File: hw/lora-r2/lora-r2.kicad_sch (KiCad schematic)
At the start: 5 parts, among them J3 Conn_02x12_Odd_Even

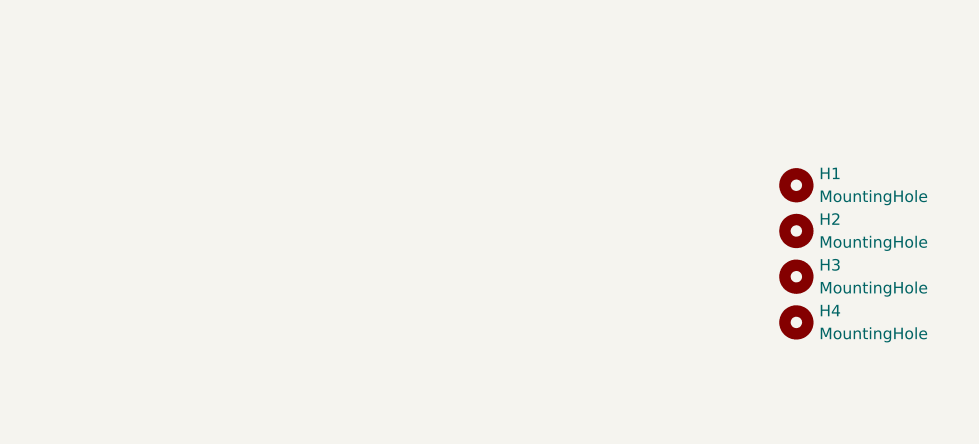
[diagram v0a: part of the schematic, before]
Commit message: Generated first Gerbers
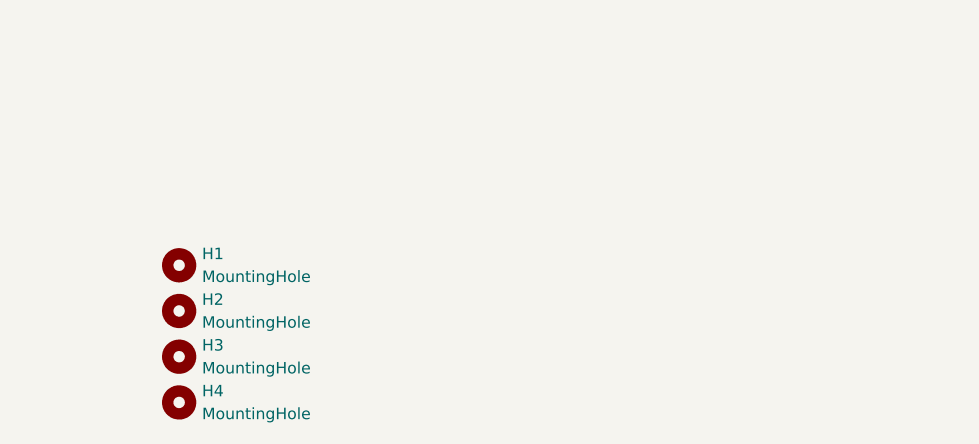
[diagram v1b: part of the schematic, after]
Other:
- company: (none) -> Bruce MacKinnon
- title: (none) -> KC1FSZ LoRa Controller Board
- moved on the sheet: H1, H2, H3, H4
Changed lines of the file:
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@@
 	(generator "eeschema")
 	(generator_version "9.0")
-	(paper "A4")
+	(paper "USLetter")
+	(title_block
+		(title "KC1FSZ LoRa Controller Board")
+		(date "2025-05-08")
+		(rev "1")
+		(company "Bruce MacKinnon")
+		(comment 1 "Copyright (C) 2025, Bruce MacKinnon")
+		(comment 2 "NOT FOR COMMERCIAL USE")
+	)
 	(junction
 		(at 107.95 102.87)
@@
 	(symbol
 		(lib_id "Mechanical:MountingHole")
-		(at 261.62 105.41 0)
+		(at 193.04 114.3 0)
 		(unit 1)
 		(exclude_from_sim yes)
@@
 		(fields_autoplaced yes)
 		(property "Reference" "H4"
-			(at 264.16 104.1399 0)
+			(at 195.58 113.0299 0)
 			(effects
 				(font
@@
 		)
 		(property "Value" "MountingHole"
-			(at 264.16 106.6799 0)
+			(at 195.58 115.5699 0)
 			(effects
 				(font
@@
 		)
 		(property "Footprint" "MountingHole:MountingHole_3.5mm"
-			(at 261.62 105.41 0)
+			(at 193.04 114.3 0)
 			(effects
 				(font
@@
 		)
 		(property "Datasheet" "~"
-			(at 261.62 105.41 0)
+			(at 193.04 114.3 0)
 			(effects
 				(font
@@
 		)
 		(property "Description" "Mounting Hole without connection"
-			(at 261.62 105.41 0)
+			(at 193.04 114.3 0)
 			(effects
 				(font
@@
 	(symbol
 		(lib_id "Mechanical:MountingHole")
-		(at 261.62 100.33 0)
+		(at 193.04 109.22 0)
 		(unit 1)
 		(exclude_from_sim yes)
@@
 		(fields_autoplaced yes)
 		(property "Reference" "H3"
-			(at 264.16 99.0599 0)
+			(at 195.58 107.9499 0)
 			(effects
 				(font
@@
 		)
 		(property "Value" "MountingHole"
-			(at 264.16 101.5999 0)
+			(at 195.58 110.4899 0)
 			(effects
 				(font
@@
 		)
 		(property "Footprint" "MountingHole:MountingHole_3.5mm"
-			(at 261.62 100.33 0)
+			(at 193.04 109.22 0)
 			(effects
 				(font
@@
 		)
 		(property "Datasheet" "~"
-			(at 261.62 100.33 0)
+			(at 193.04 109.22 0)
 			(effects
 				(font
@@
 		)
 		(property "Description" "Mounting Hole without connection"
-			(at 261.62 100.33 0)
+			(at 193.04 109.22 0)
 			(effects
 				(font
@@
 	(symbol
 		(lib_id "Mechanical:MountingHole")
-		(at 261.62 95.25 0)
+		(at 193.04 104.14 0)
 		(unit 1)
 		(exclude_from_sim yes)
@@
 		(fields_autoplaced yes)
 		(property "Reference" "H2"
-			(at 264.16 93.9799 0)
+			(at 195.58 102.8699 0)
 			(effects
 				(font
@@
 		)
 		(property "Value" "MountingHole"
-			(at 264.16 96.5199 0)
+			(at 195.58 105.4099 0)
 			(effects
 				(font
@@
 		)
 		(property "Footprint" "MountingHole:MountingHole_3.5mm"
-			(at 261.62 95.25 0)
+			(at 193.04 104.14 0)
 			(effects
 				(font
@@
 		)
 		(property "Datasheet" "~"
-			(at 261.62 95.25 0)
+			(at 193.04 104.14 0)
 			(effects
 				(font
@@
 		)
 		(property "Description" "Mounting Hole without connection"
-			(at 261.62 95.25 0)
+			(at 193.04 104.14 0)
 			(effects
 				(font
@@
 	(symbol
 		(lib_id "Mechanical:MountingHole")
-		(at 261.62 90.17 0)
+		(at 193.04 99.06 0)
 		(unit 1)
 		(exclude_from_sim yes)
@@
 		(fields_autoplaced yes)
 		(property "Reference" "H1"
-			(at 264.16 88.8999 0)
+			(at 195.58 97.7899 0)
 			(effects
 				(font
@@
 		)
 		(property "Value" "MountingHole"
-			(at 264.16 91.4399 0)
+			(at 195.58 100.3299 0)
 			(effects
 				(font
@@
 		)
 		(property "Footprint" "MountingHole:MountingHole_3.5mm"
-			(at 261.62 90.17 0)
+			(at 193.04 99.06 0)
 			(effects
 				(font
@@
 		)
 		(property "Datasheet" "~"
-			(at 261.62 90.17 0)
+			(at 193.04 99.06 0)
 			(effects
 				(font
@@
 		)
 		(property "Description" "Mounting Hole without connection"
-			(at 261.62 90.17 0)
-			(effects
-				(font
+			(at 193.04 99.06 0)
+			(effects
+				(font

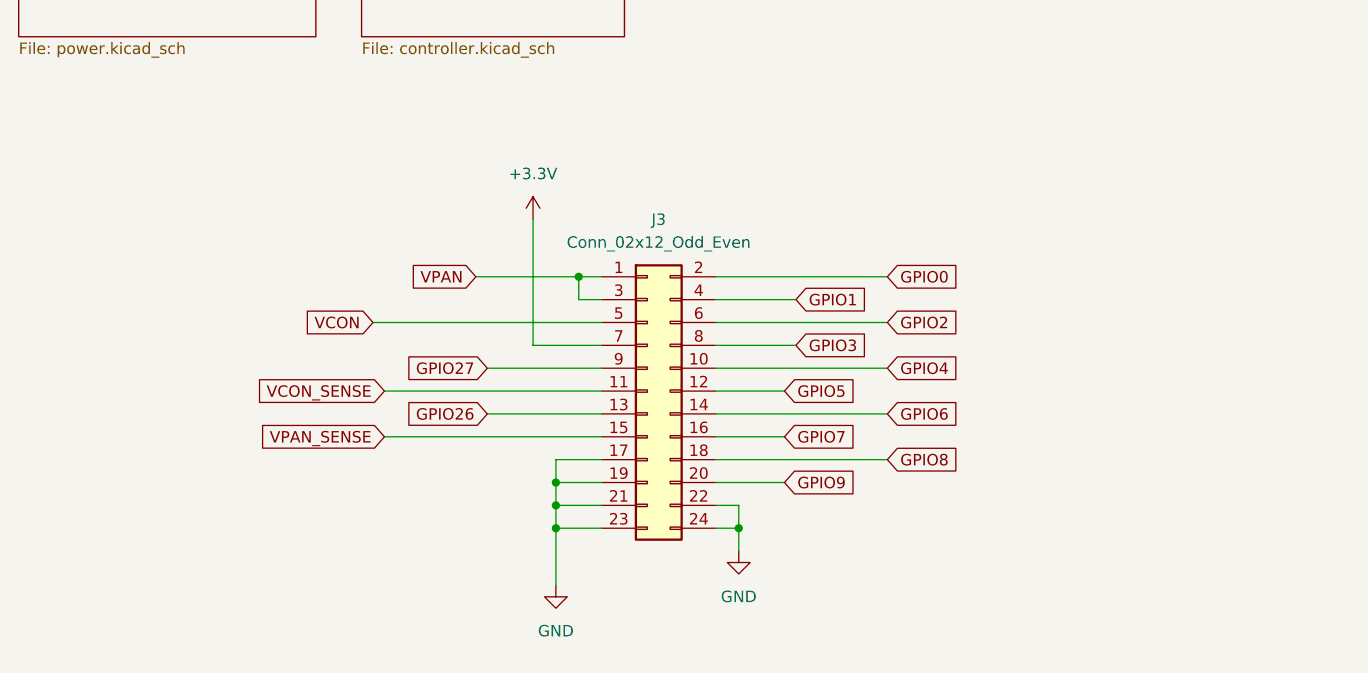
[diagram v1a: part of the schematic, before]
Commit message: SENT TO FAB (2025-05-08 13:04)
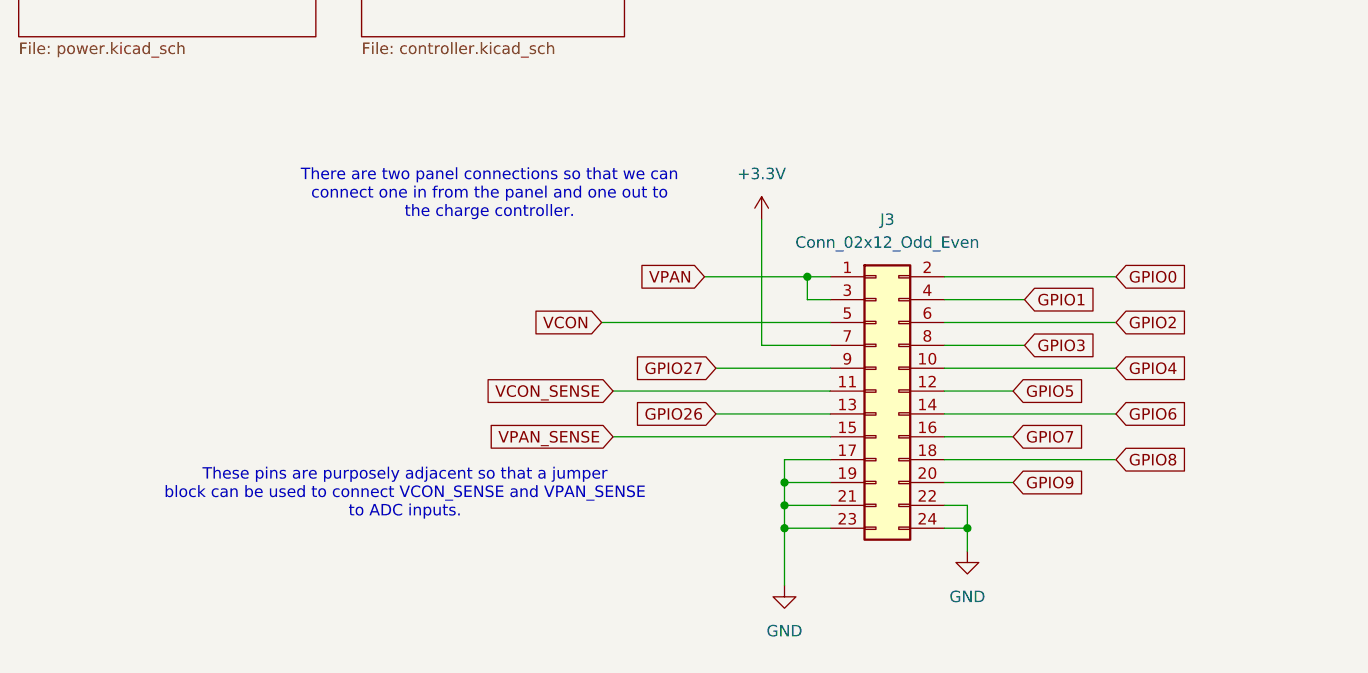
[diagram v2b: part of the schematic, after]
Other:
- note added: "There are two panel connections so that we can connect one in from the panel and one out to the charge controller."
- note added: "These pins are purposely adjacent so that a jumper block can be used to connect VCON_SENSE and VPAN_SENSE to ADC inputs."
- moved on the sheet: J3
